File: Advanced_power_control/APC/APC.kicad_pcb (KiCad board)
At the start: 4 copper layers, 59.5 x 71.5 mm, 51 parts, among them J1 AVR-JTAG-10, J10 CMD_IN, J11 PWR_V_SEL, J12 12/24 V_IN, J13 220_OUT, J2 EM_STOP_INT, J3 STATUS_LED, J4 EM_STOP, J5 PWR_BTN, J6 POWER_LED, J7 220 IN, J8 CMD_OUT, J9 CMD_V_SEL, K1 G5LE-1, Q1 IRLML0030, Q2 IRLML0030, Q3 IRLML0030, U1 ATmega164PA-AU, U2 LTV-817, U3 LTV-817, U4 LTV-817

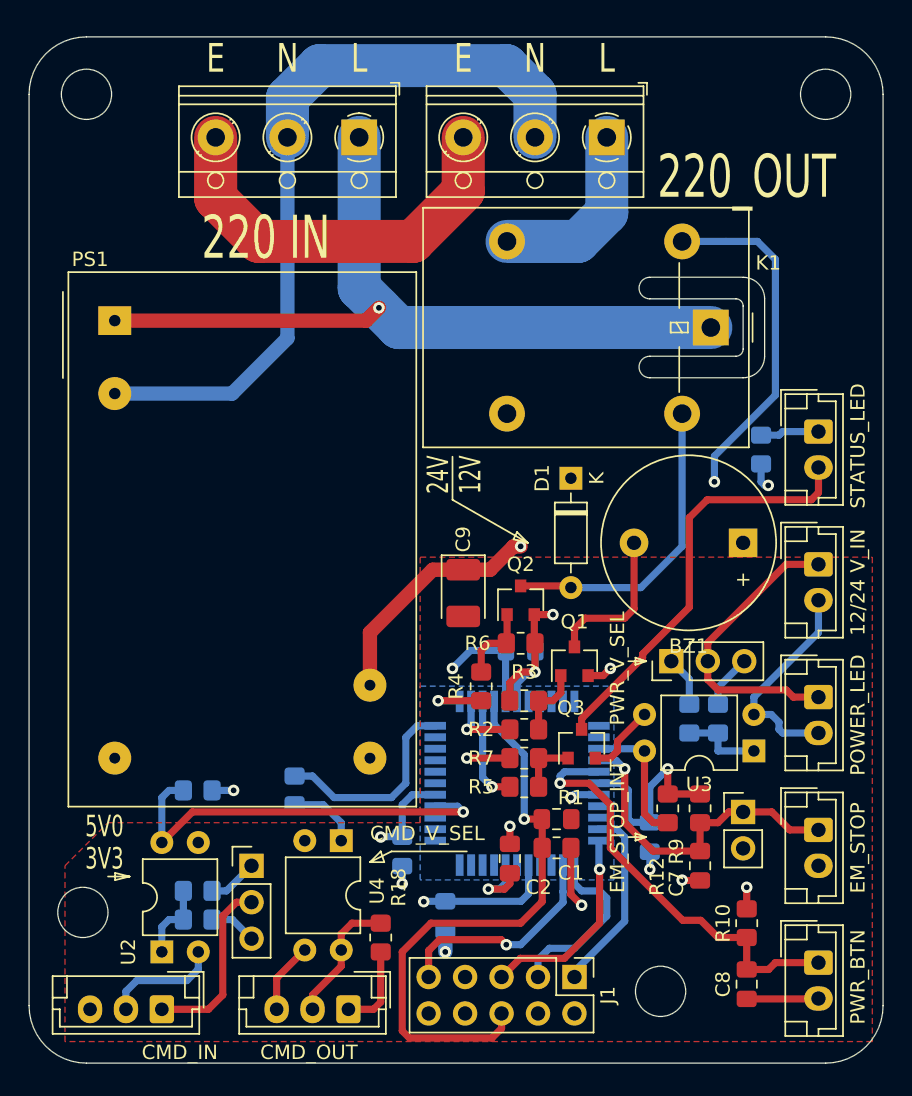
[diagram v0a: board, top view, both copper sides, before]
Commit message: Update APC.kicad_pcb
PreFinal correction
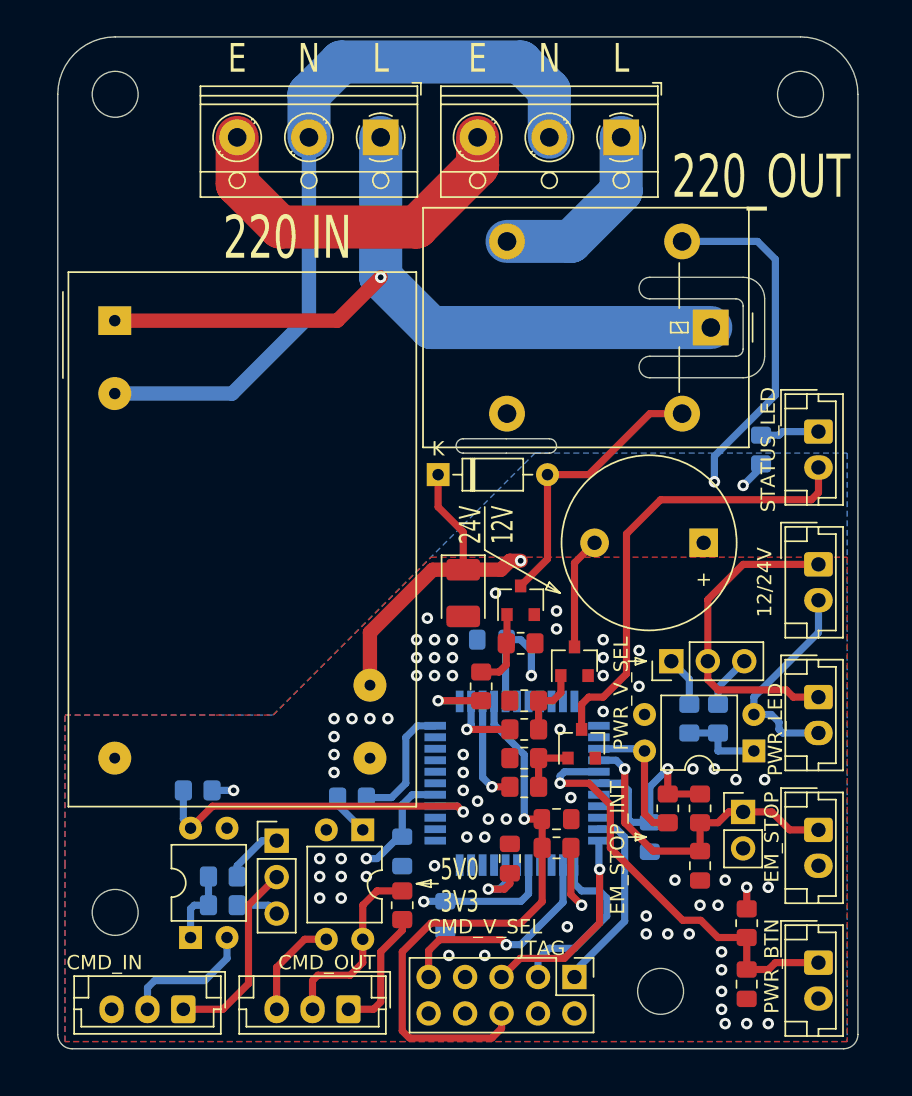
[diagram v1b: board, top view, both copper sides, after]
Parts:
- J12: value 12/24 V_IN -> 12/24V
- J6: value POWER_LED -> PWR_LED
- moved D1 9.25 mm to (114.8, 60.5), turned to 0 degrees
- moved R13 4.03 mm to (108.8, 83.0), turned to 0 degrees
- moved BZ1 2.75 mm to (133.2, 65.2)
- moved R18 2.70 mm to (112.2, 90.5)
- moved J9 2.47 mm to (103.5, 86.0)
- moved U2 2.24 mm to (97.5, 92.8)
- moved C3 2.14 mm to (118.5, 72.0), turned to 0 degrees
- moved R14 2.02 mm to (99.8, 90.5)
- moved R15 2.02 mm to (99.8, 88.5)
- moved U4 1.68 mm to (109.5, 85.2)
- moved J10 1.50 mm to (97.0, 97.8)
- moved J7 1.50 mm to (110.8, 37.0)
- moved J13 1.00 mm to (127.5, 37.0)
- renumbered J1 to JTAG
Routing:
- net GND: track 36.3 -> 0.00 mm, vias 10 -> 67
- net +5V: track 87.8 -> 96.9 mm
- net /CMD_OUT: track 14.4 -> 8.75 mm
- net /CMD_IN: track 29.0 -> 24.8 mm
- net /S: track 9.14 -> 13.2 mm
- net /E: track 27.9 -> 25.0 mm
- net /V: track 5.96 -> 8.83 mm
- net Net-(BZ1-Pad2): track 10.6 -> 7.83 mm
- net Net-(J3-Pad2): track 29.3 -> 31.8 mm
- net /G: track 4.94 -> 7.19 mm
- net /P_ON: track 21.7 -> 19.7 mm
- net Net-(R13-Pad1): track 5.02 -> 2.97 mm
- net /V_SEL: track 20.8 -> 22.5 mm
- net Net-(J10-Pad2): track 8.14 -> 9.34 mm
- net /CMD_V_IN: track 12.6 -> 13.5 mm
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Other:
- board size 59.5 x 71.5 mm -> 55.8 x 70.5 mm
